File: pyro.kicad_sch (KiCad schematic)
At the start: 34 parts, among them J15 DB141R-2.54-8P-GN, Q1 MJD44H11T4G, Q10 PJM09P30DF, Q11 PJM09P30DF, Q12 PJM09P30DF, Q13 PJM09P30DF, Q4 BC817-25,215, Q5 NMOS, Q6 NMOS, Q7 NMOS, Q8 NMOS, Q9 NMOS, U7 LM334M

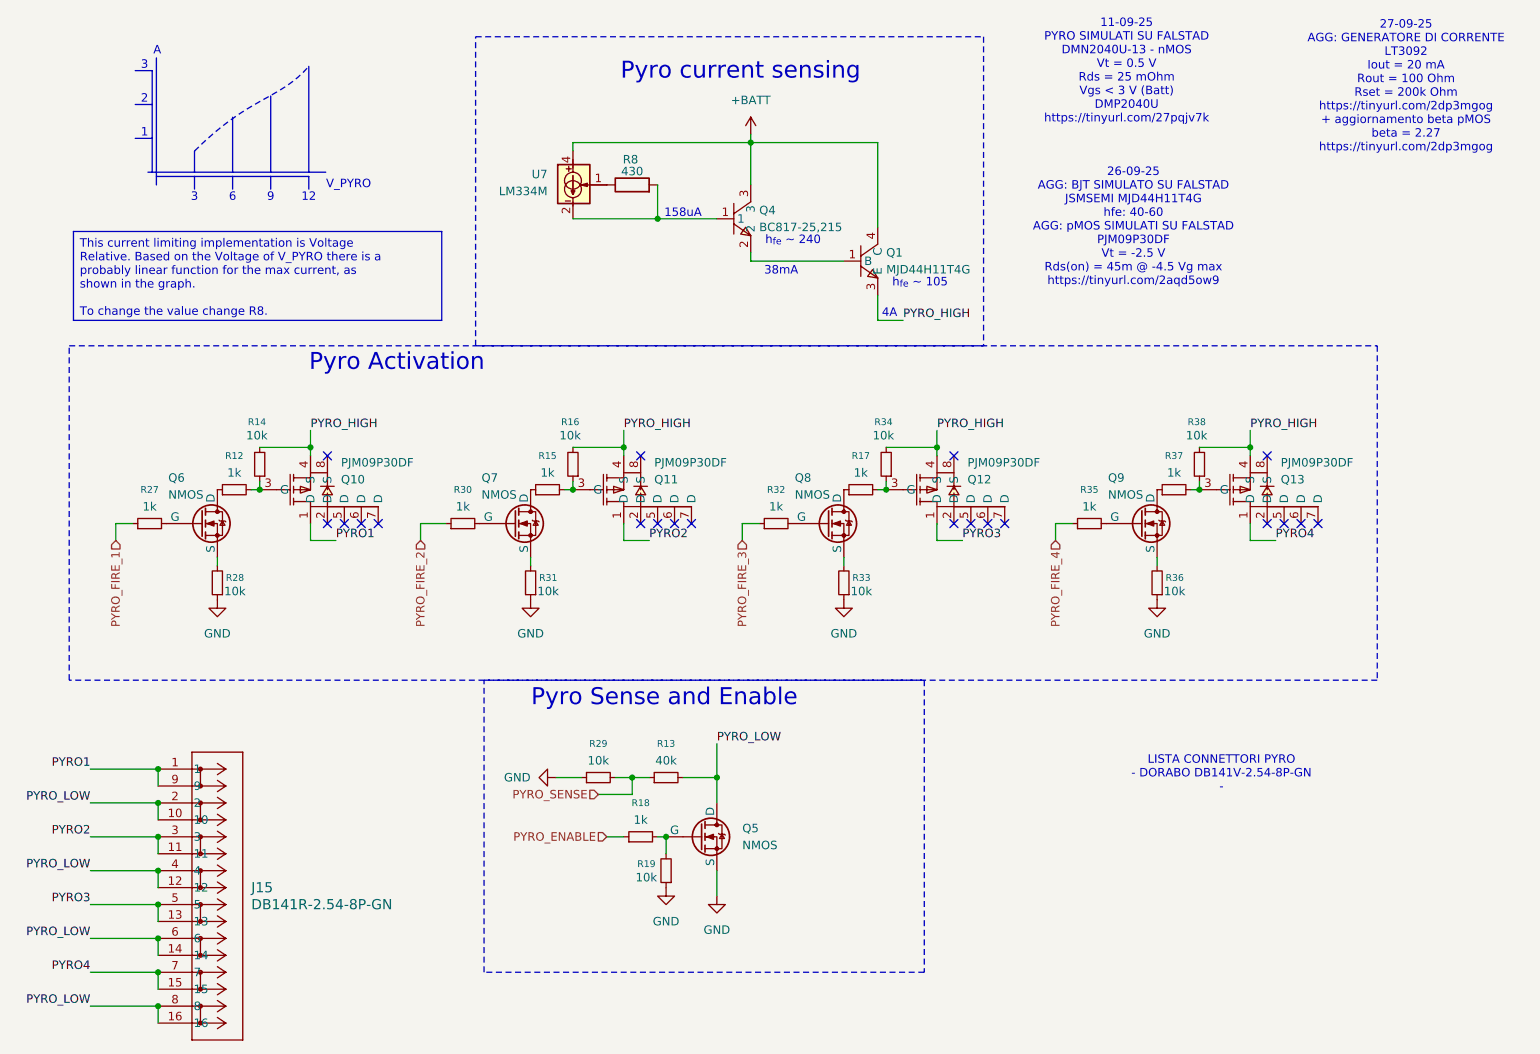
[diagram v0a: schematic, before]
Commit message: perché non funziona
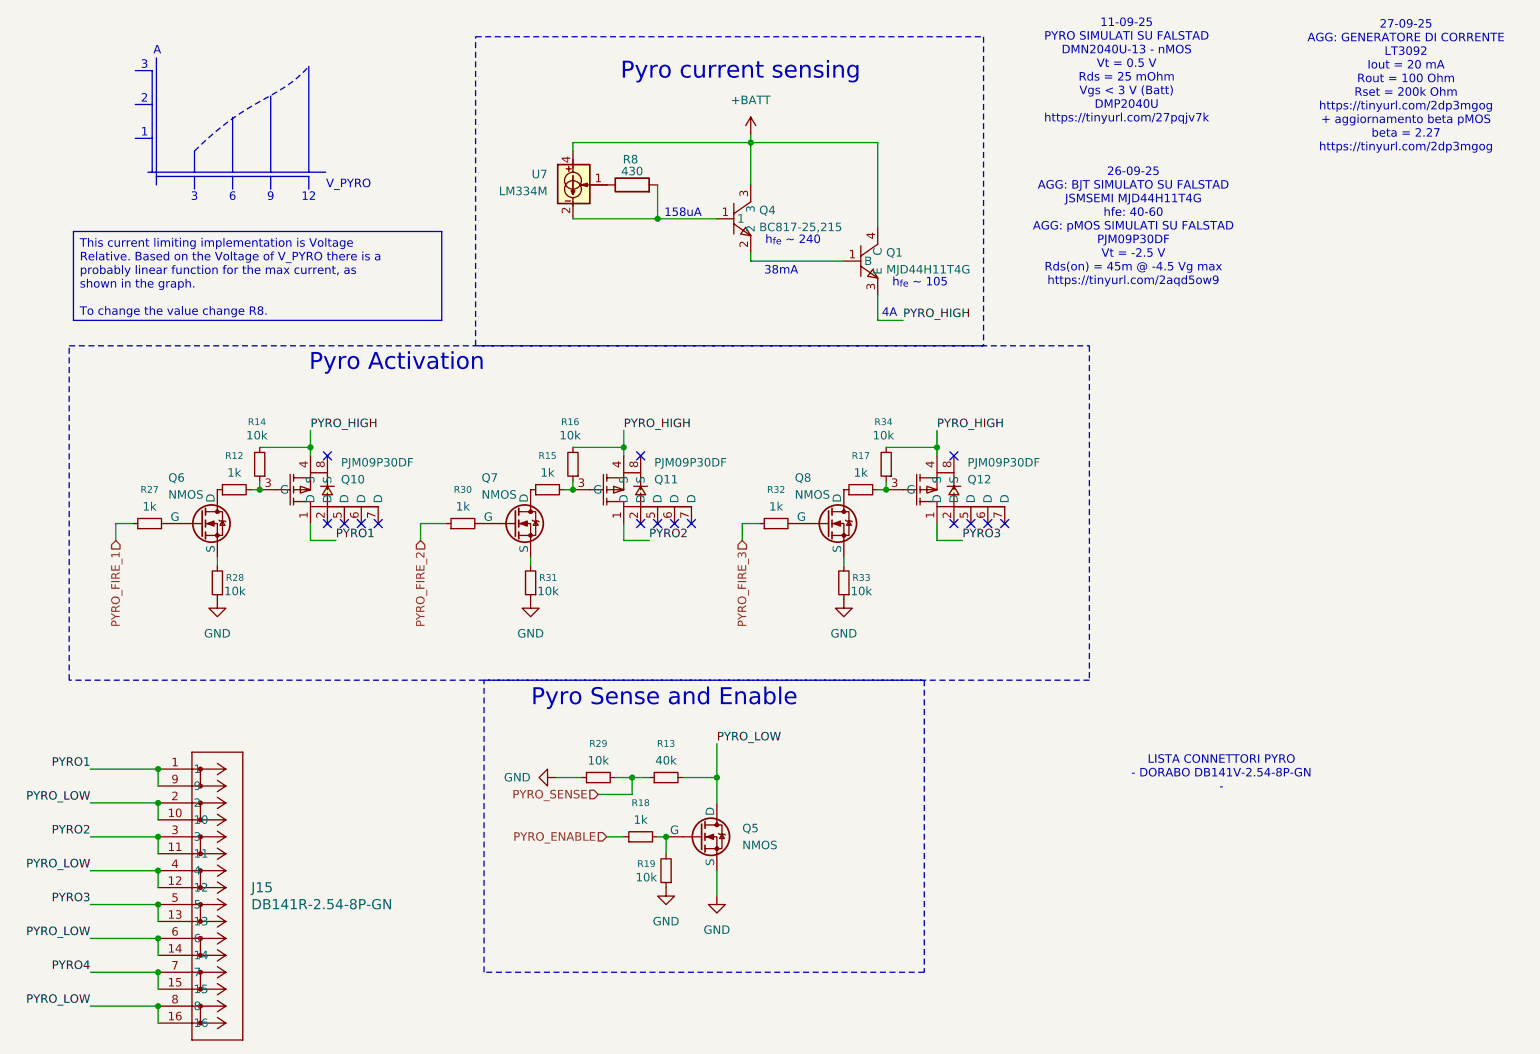
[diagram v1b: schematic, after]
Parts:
- removed Q13: PJM09P30DF, easyeda2kicad:DFN-6_L2.0-W2.0-P0.65-BL-EP-1, symbol WF5803F:PJM09P30DF
- removed Q9: NMOS, Package_TO_SOT_SMD:SOT-23_Handsoldering, symbol Simulation_SPICE:NMOS
- removed R35, R37: 1k, Resistor_SMD:R_0603_1608Metric_Pad0.98x0.95mm_HandSolder, symbol Device:R_Small
- removed R36, R38: 10k, Resistor_SMD:R_0603_1608Metric_Pad0.98x0.95mm_HandSolder, symbol Device:R_Small
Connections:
- no-connect marks 20 -> 15
